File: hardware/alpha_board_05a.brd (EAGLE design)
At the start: 85.1 x 74.9 mm, 18 parts

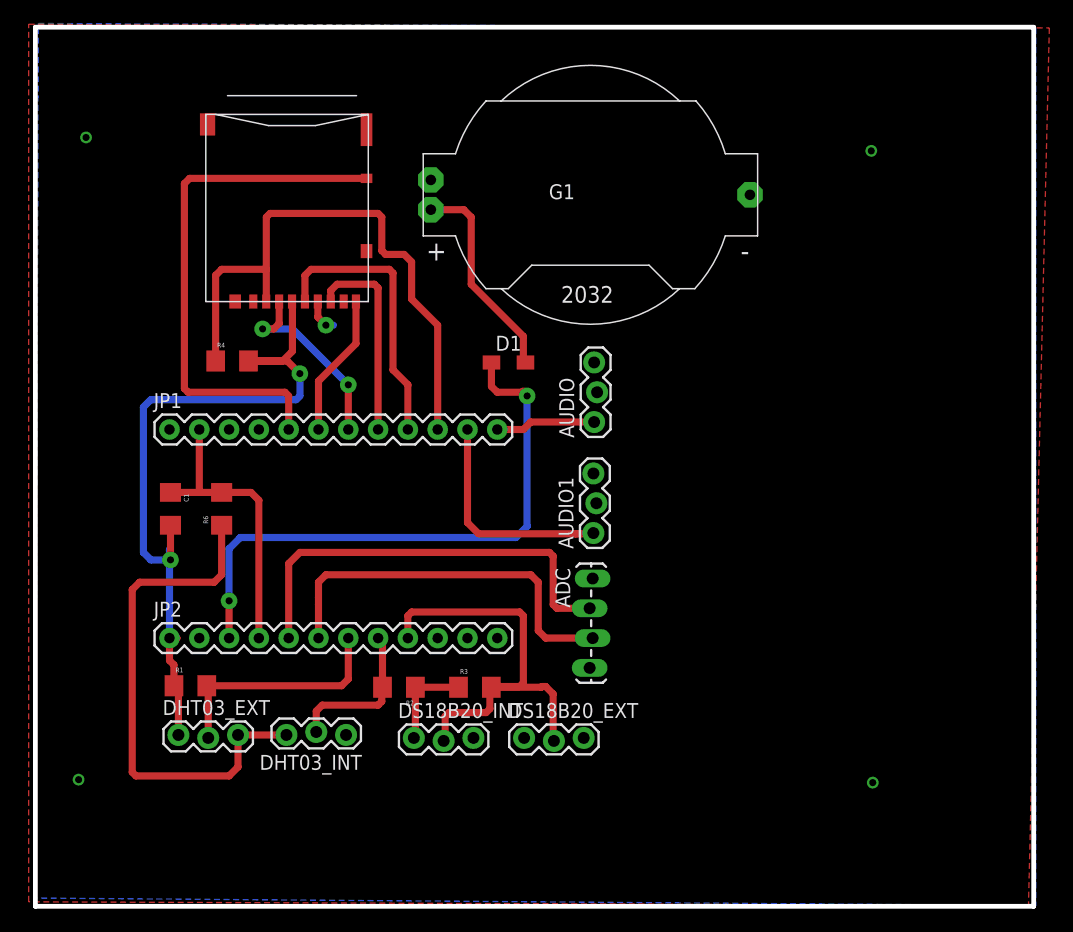
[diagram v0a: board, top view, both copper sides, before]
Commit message: few bug changes
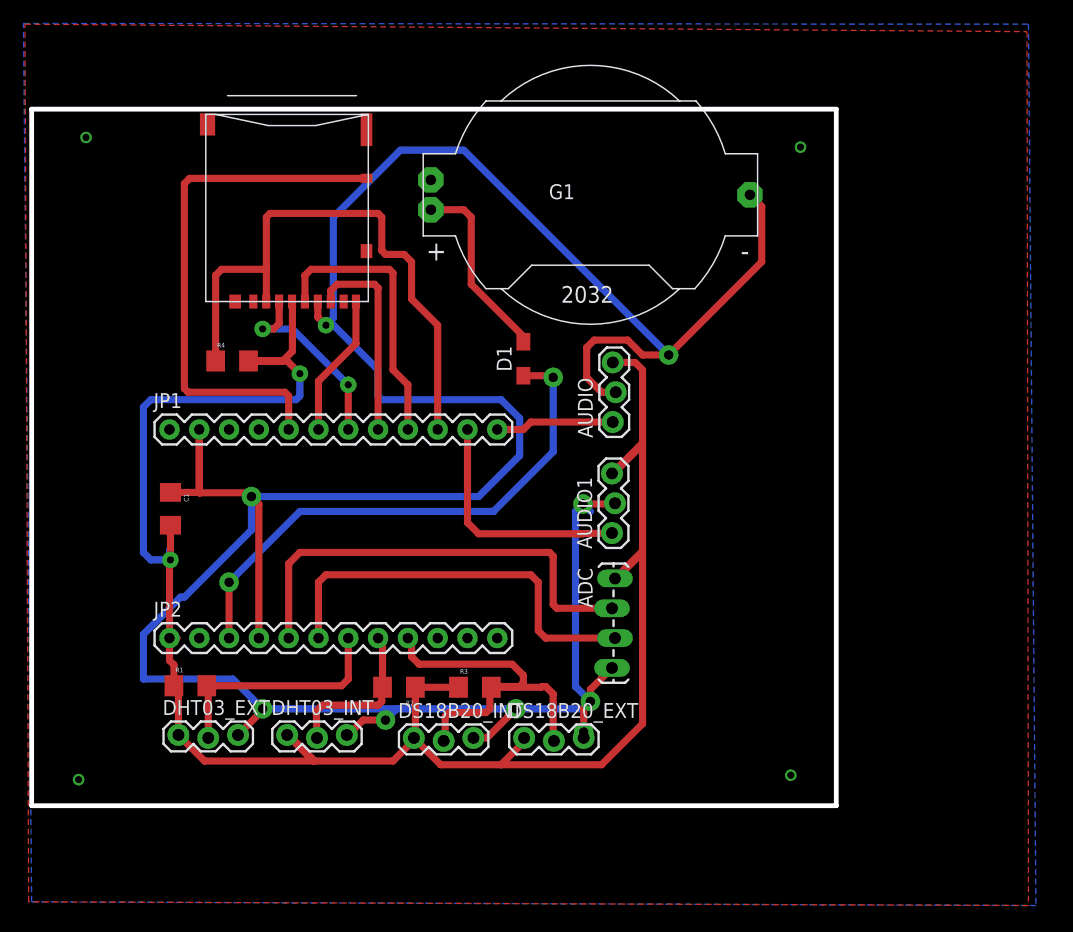
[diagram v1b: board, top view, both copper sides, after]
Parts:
- removed R6: 0, SparkFun:1206
- moved DHT03_INT 5.02 mm to (16.4, 13.2), turned to 0 degrees
- moved ADC 1.91 mm to (44.3, 26.7)
- moved AUDIO 1.59 mm to (44.3, 40.0)
- moved AUDIO1 1.59 mm to (44.2, 30.5)
- moved D1 1.31 mm to (36.5, 45.4), turned to 90 degrees
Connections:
- removed net GNDR: DHT03_EXT.3, DHT03_INT.3, R6.1
- net GND: now also DHT03_EXT.3, DHT03_INT.3; no longer R6.2
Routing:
- net GND: track 27.9 -> 260.9 mm, vias 1 -> 9
- net VCC: track 72.9 -> 172.0 mm
- net GNDR: track 44.2 -> 0.00 mm
- net D3: track 38.4 -> 33.2 mm
- net VDDA: track 50.3 -> 45.9 mm
- net D7: track 36.8 -> 38.7 mm
- net D6: track 33.0 -> 35.0 mm
- net N$3: track 18.0 -> 16.2 mm
- net N$2: track 8.52 -> 10.1 mm
- net N$6: track 19.7 -> 21.3 mm
- net D4: track 14.0 -> 14.5 mm
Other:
- board size 85.1 x 74.9 mm -> 68.6 x 59.4 mm
